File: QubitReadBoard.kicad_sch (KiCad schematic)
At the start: 0 parts

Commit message: Selected room temp amp
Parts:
- added U1: HMC8411LP2FE, CP_6_12_ADI, symbol HMC8411LP2FE:HMC8411LP2FE
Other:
- title: (none) -> Qubit Readout Board
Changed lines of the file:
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@@
 	(generator_version "10.0")
 	(paper "A4")
+	(title_block
+		(title "Qubit Readout Board")
+		(date "2026-08-18")
+	)
+	(symbol
+		(lib_id "HMC8411LP2FE:HMC8411LP2FE")
+		(at 48.26 101.6 0)
+		(unit 1)
+		(body_style 1)
+		(exclude_from_sim no)
+		(in_bom yes)
+		(on_board yes)
+		(in_pos_files yes)
+		(dnp no)
+		(fields_autoplaced yes)
+		(property "Reference" "U1"
+			(at 73.66 91.44 0)
+			(show_name no)
+			(do_not_autoplace no)
+			(effects
+				(font
+					(size 1.524 1.524)
+				)
+			)
+		)
+		(property "Value" "HMC8411LP2FE"
+			(at 73.66 93.98 0)
+			(show_name no)
+			(do_not_autoplace no)
+			(effects
+				(font
+					(size 1.524 1.524)
+				)
+			)
+		)
+		(property "Footprint" "CP_6_12_ADI"
+			(at 48.26 101.6 0)
+			(hide yes)
+			(show_name no)
+			(do_not_autoplace no)
+			(effects
+				(font
+					(size 1.27 1.27)
+					(italic yes)
+				)
+			)
+		)
+		(property "Datasheet" "https://www.analog.com/media/en/technical-documentation/data-sheets/HMC8411LP2FE.pdf"
+			(at 48.26 101.6 0)
+			(hide yes)
+			(show_name no)
+			(do_not_autoplace no)
+			(effects
+				(font
+					(size 1.27 1.27)
+					(italic yes)
+				)
+			)
+		)
+		(property "Description" ""
+			(at 48.26 101.6 0)
+			(hide yes)
+			(show_name no)
+			(do_not_autoplace no)
+			(effects
+				(font
+					(size 1.27 1.27)
+				)
+			)
+		)
+		(pin "2"
+		)
+		(pin "1"
+		)
+		(pin "5"
+		)
+		(pin "7"
+		)
+		(pin "4"
+		)
+		(pin "3"
+		)
+		(pin "6"
+		)
+		(instances
+			(project "QubitReadBoard"
+				(path "/56824d00-9c24-4fa5-a72f-e9b9506cb609"
+					(reference "U1")
+					(unit 1)
+				)
+			)
+		)
+	)
 	(sheet_instances
 		(path "/"

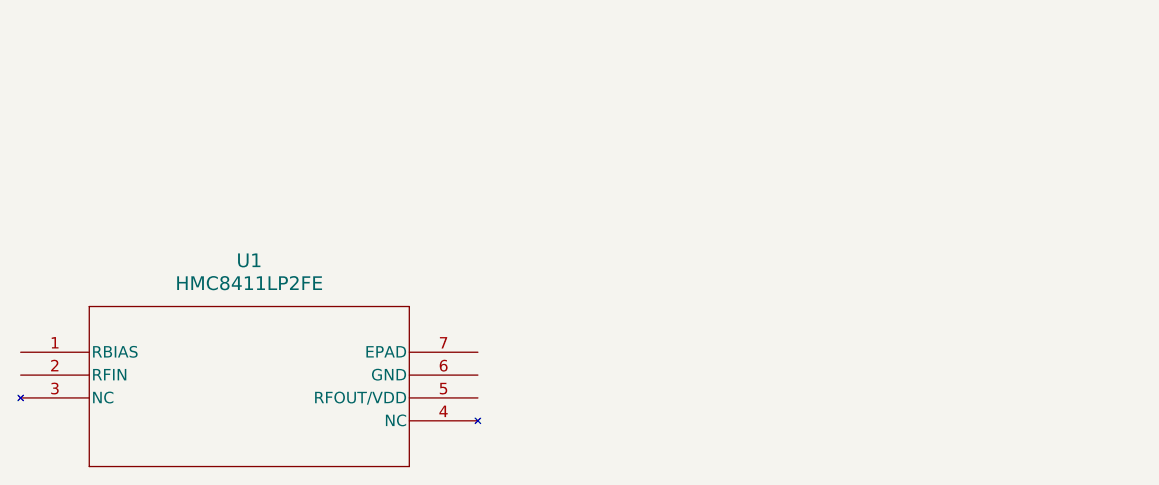
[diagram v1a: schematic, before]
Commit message: Added mixer
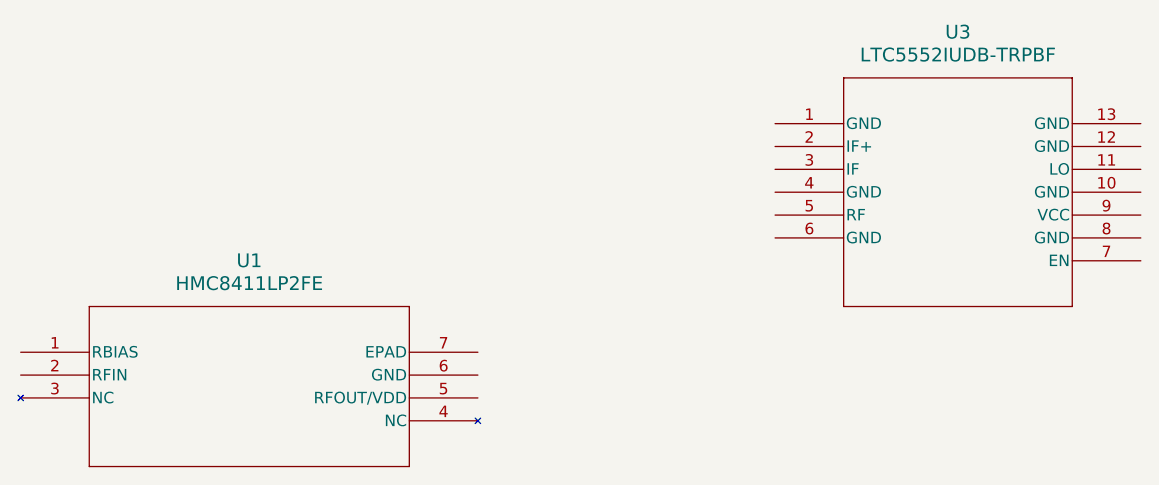
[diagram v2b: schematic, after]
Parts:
- added U3: LTC5552IUDB-TRPBF, UDB_12_ADI, symbol LTC5552:LTC5552IUDB-TRPBF
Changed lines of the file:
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@@
 	(title_block
 		(title "Qubit Readout Board")
-		(date "2026-08-18")
+		(date "2026-08-19")
 	)
 	(symbol
+		(lib_id "LTC5552:LTC5552IUDB-TRPBF")
+		(at 132.08 76.2 0)
+		(unit 1)
+		(body_style 1)
+		(exclude_from_sim no)
+		(in_bom yes)
+		(on_board yes)
+		(in_pos_files yes)
+		(dnp no)
+		(fields_autoplaced yes)
+		(property "Reference" "U3"
+			(at 152.4 66.04 0)
+			(show_name no)
+			(do_not_autoplace no)
+			(effects
+				(font
+					(size 1.524 1.524)
+				)
+			)
+		)
+		(property "Value" "LTC5552IUDB-TRPBF"
+			(at 152.4 68.58 0)
+			(show_name no)
+			(do_not_autoplace no)
+			(effects
+				(font
+					(size 1.524 1.524)
+				)
+			)
+		)
+		(property "Footprint" "UDB_12_ADI"
+			(at 132.08 76.2 0)
+			(hide yes)
+			(show_name no)
+			(do_not_autoplace no)
+			(effects
+				(font
+					(size 1.27 1.27)
+					(italic yes)
+				)
+			)
+		)
+		(property "Datasheet" "https://www.analog.com/media/en/technical-documentation/data-sheets/5552f.pdf"
+			(at 132.08 76.2 0)
+			(hide yes)
+			(show_name no)
+			(do_not_autoplace no)
+			(effects
+				(font
+					(size 1.27 1.27)
+					(italic yes)
+				)
+			)
+		)
+		(property "Description" ""
+			(at 132.08 76.2 0)
+			(hide yes)
+			(show_name no)
+			(do_not_autoplace no)
+			(effects
+				(font
+					(size 1.27 1.27)
+				)
+			)
+		)
+		(pin "9"
+		)
+		(pin "11"
+		)
+		(pin "8"
+		)
+		(pin "1"
+		)
+		(pin "7"
+		)
+		(pin "3"
+		)
+		(pin "4"
+		)
+		(pin "6"
+		)
+		(pin "2"
+		)
+		(pin "5"
+		)
+		(pin "10"
+		)
+		(pin "12"
+		)
+		(pin "13"
+		)
+		(instances
+			(project "QubitReadBoard"
+				(path "/56824d00-9c24-4fa5-a72f-e9b9506cb609"
+					(reference "U3")
+					(unit 1)
+				)
+			)
+		)
+	)
+	(symbol
